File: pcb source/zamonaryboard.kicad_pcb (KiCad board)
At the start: 2 copper layers, 52.3 x 40.6 mm, 19 parts, among them J1 USB_C_Receptacle_USB2.0_14P, SW1 SW_Push, U1 ESP32-S2, U2 ME6211C33M5, Y1 Crystal_GND24

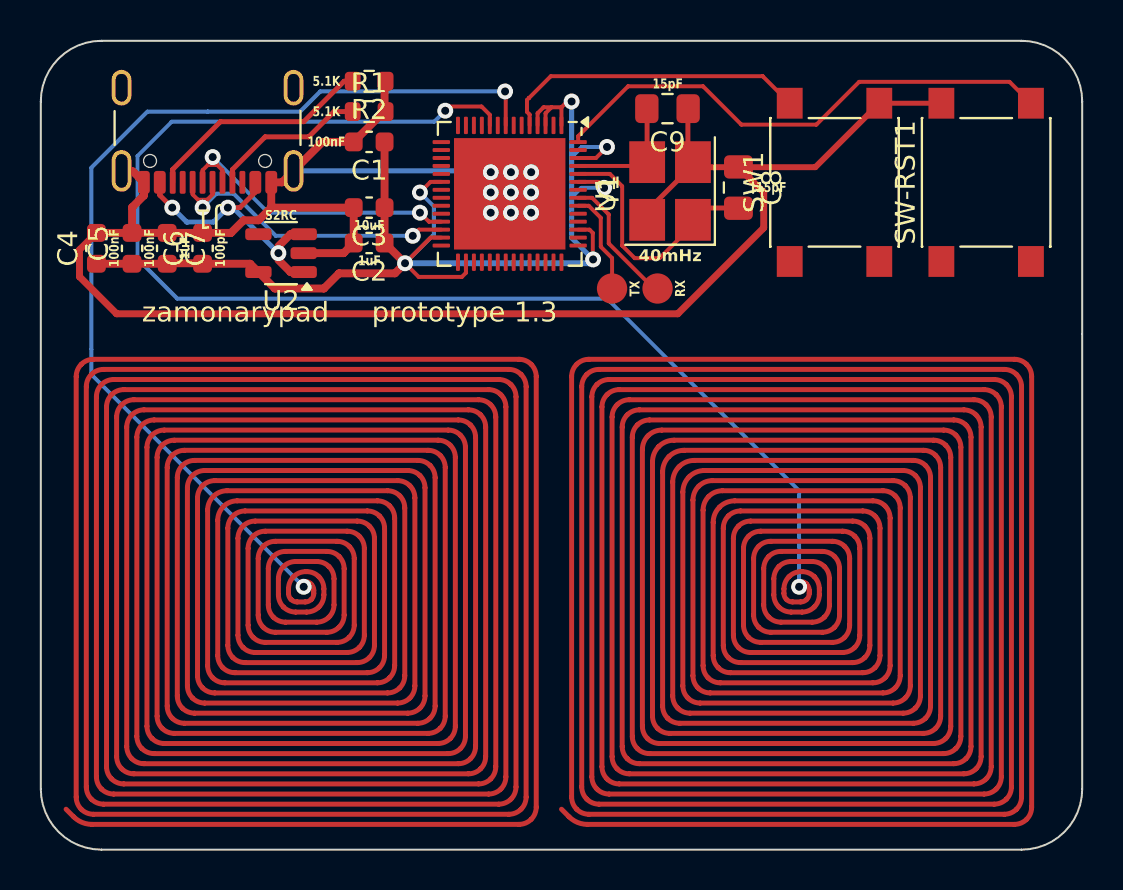
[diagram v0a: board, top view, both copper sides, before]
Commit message: exported gerber files for prototype 1.3, cleanup
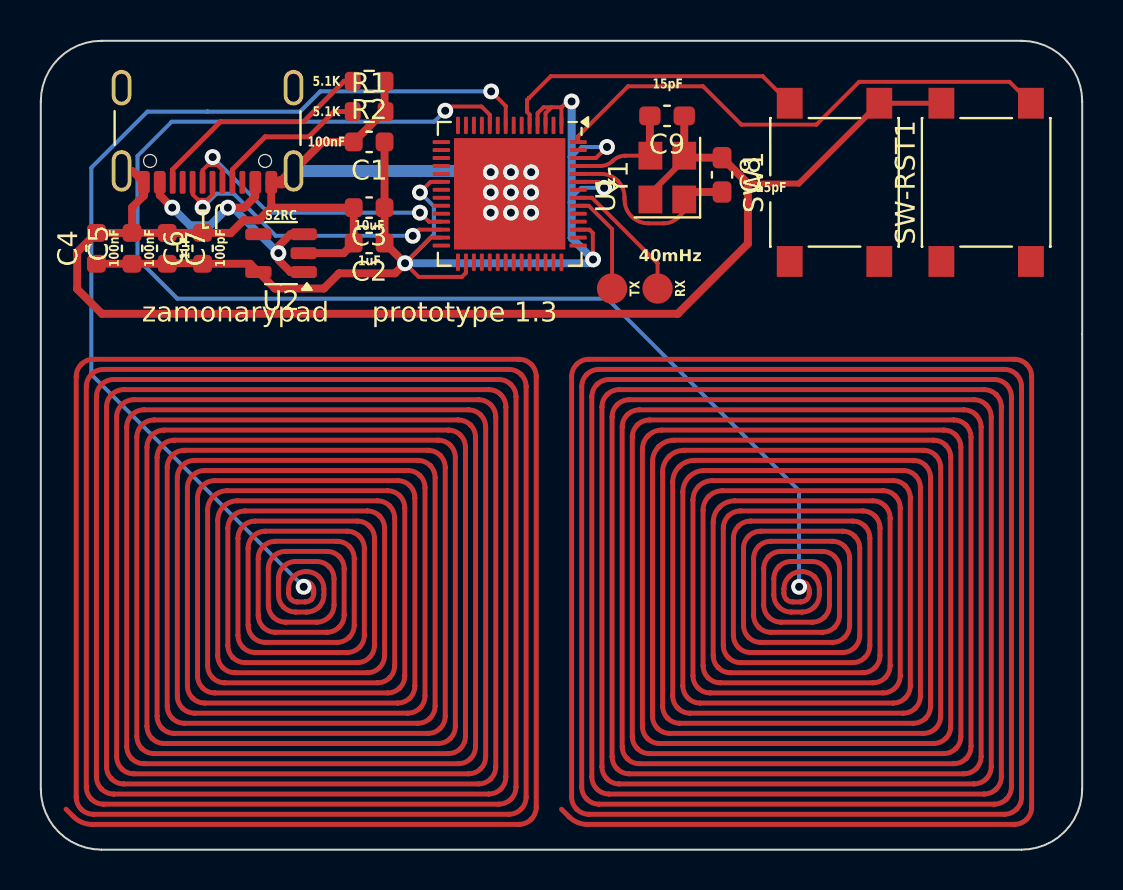
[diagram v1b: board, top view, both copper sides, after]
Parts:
- C8, C9: footprint Capacitor_SMD:C_0805_2012Metric_Pad1.18x1.45mm_HandSolder -> Capacitor_SMD:C_0603_1608Metric_Pad1.08x0.95mm_HandSolder
- Y1: footprint Crystal:Crystal_SMD_3225-4Pin_3.2x2.5mm_HandSoldering -> Crystal:Crystal_SMD_3225-4Pin_3.2x2.5mm
- moved C8 1.04 mm to (153.1, 78.4)
- moved Y1 0.69 mm to (150.3, 78.5)
- moved C9 0.36 mm to (150.3, 75.4)
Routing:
- net GND: track 119.8 -> 105.5 mm
- net Net-(U1-XTAL_N): track 13.1 -> 9.63 mm
- net Net-(U1-XTAL_P): track 6.39 -> 5.77 mm
